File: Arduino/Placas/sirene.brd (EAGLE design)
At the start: 57 x 51 mm, 8 parts

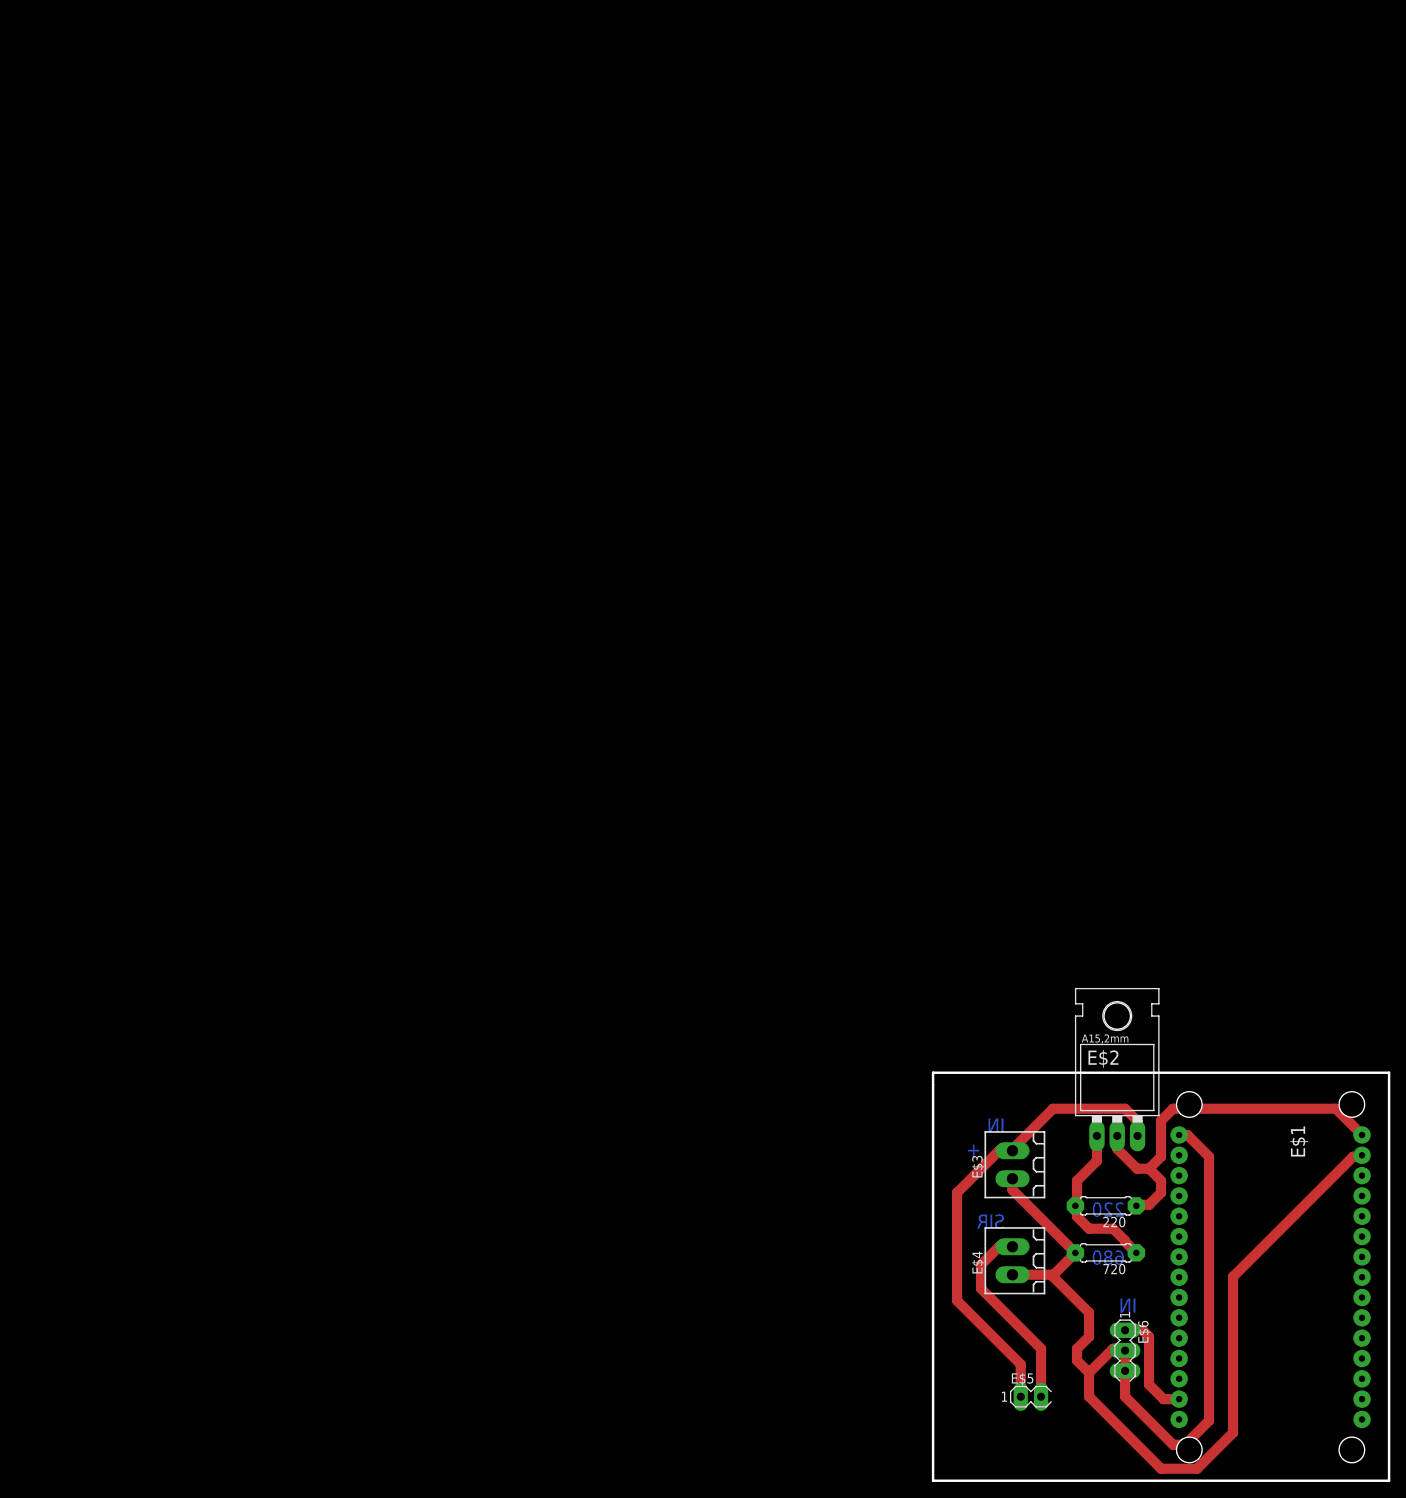
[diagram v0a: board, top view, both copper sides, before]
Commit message: Sirene board updated
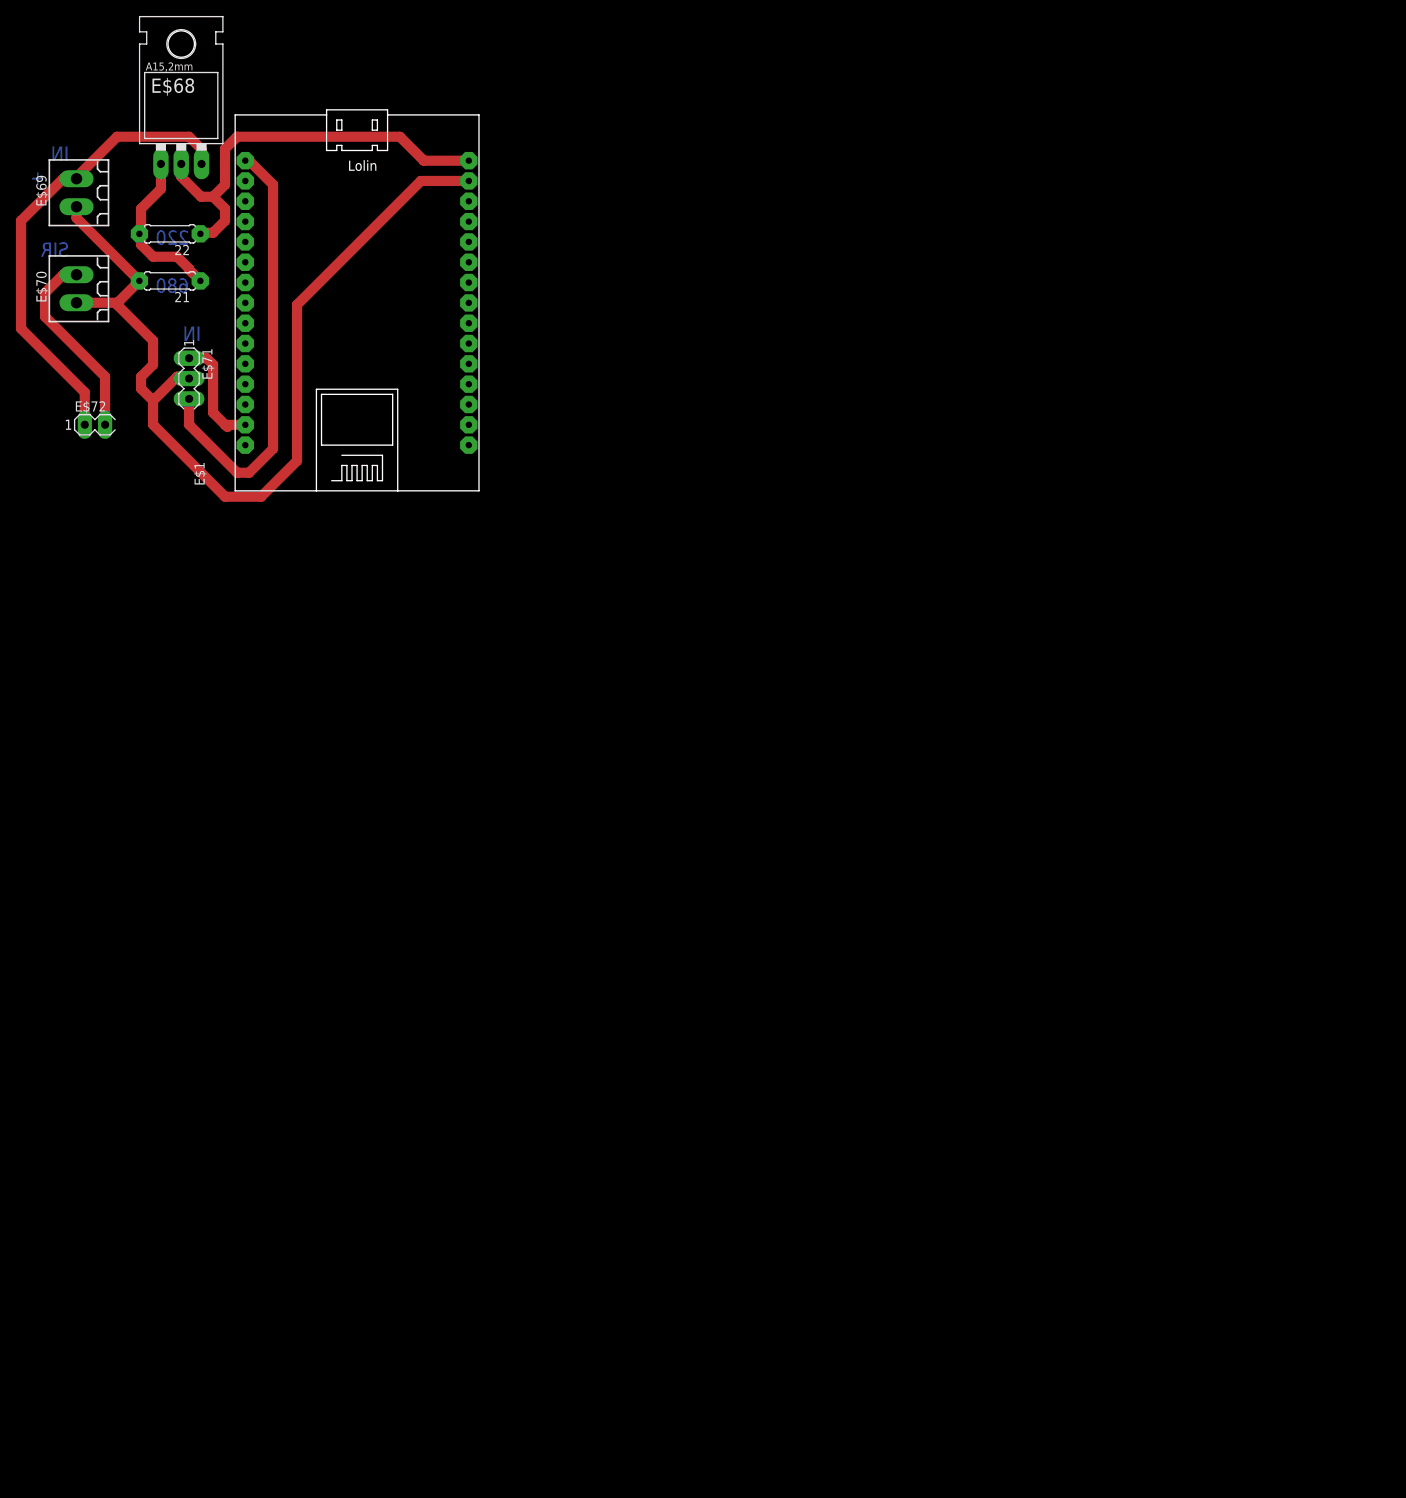
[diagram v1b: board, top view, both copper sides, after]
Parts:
- removed 220, 720: (no value), rcl:0207/7
- removed E$2: (no value), v-reg:317TL
- removed E$3, E$4: (no value), con-weidmueller-sl35:180G-2
- removed E$5: (no value), con-lstb:MA03-1
- removed E$6: (no value), con-lstb:MA04-1
- added 21, 22: (no value), rcl:0207/7
- added E$68: (no value), v-reg:317TL
- added E$69, E$70: (no value), con-weidmueller-sl35:180G-2
- added E$71: (no value), con-lstb:MA04-1
- added E$72: (no value), con-lstb:MA03-1
- E$1: device ESP12E_DEVKIT:ESP12E_DEVKIT -> Lolin:LOLIN
- moved E$1 167.9 mm to (-48.0, 166.5), turned to 90 degrees
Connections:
- removed net S$1: E$2.3, E$3.2, E$5.1
- removed net S$2: 220.1, E$1.VIN, E$2.2
- removed net S$3: 220.2, 720.1, E$2.1
- removed net S$4: E$1.3V3@2, E$6.3
- removed net S$5: E$1.D1, E$6.1
- removed net S$7: 720.2, E$1.GND@1, E$3.1, E$4.1, E$6.2
- removed net S$9: E$4.2, E$5.2
- new net S$80: E$68.3, E$69.2, E$72.1
- new net S$81: 22.1, E$1.VIN, E$68.2
- new net S$82: 21.1, 22.2, E$68.1
- new net S$83: E$70.2, E$72.2
- new net S$84: E$1.3V1, E$71.3
- new net S$85: E$1.D1, E$71.1
- new net S$86: 21.2, E$1.G2, E$69.1, E$70.1, E$71.2
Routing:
- net S$86: track 0.00 -> 116.9 mm
- net S$7: track 112.7 -> 0.00 mm
- net S$80: track 0.00 -> 58.4 mm
- net S$1: track 58.4 -> 0.00 mm
- net S$4: track 55.3 -> 0.00 mm
- net S$84: track 0.00 -> 55.2 mm
- net S$81: track 0.00 -> 53.0 mm
- net S$2: track 48.1 -> 0.00 mm
- net S$83: track 0.00 -> 24.5 mm
- net S$9: track 24.5 -> 0.00 mm
- net S$3: track 20.8 -> 0.00 mm
- net S$82: track 0.00 -> 20.8 mm
- net S$85: track 0.00 -> 14.4 mm
- net S$5: track 13.8 -> 0.00 mm
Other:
- board size 57 x 51 mm -> 30.5 x 47.6 mm
